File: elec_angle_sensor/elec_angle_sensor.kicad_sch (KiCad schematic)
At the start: 19 parts, among them J1 JST SH, J7 JST SH, U1 AS5600L

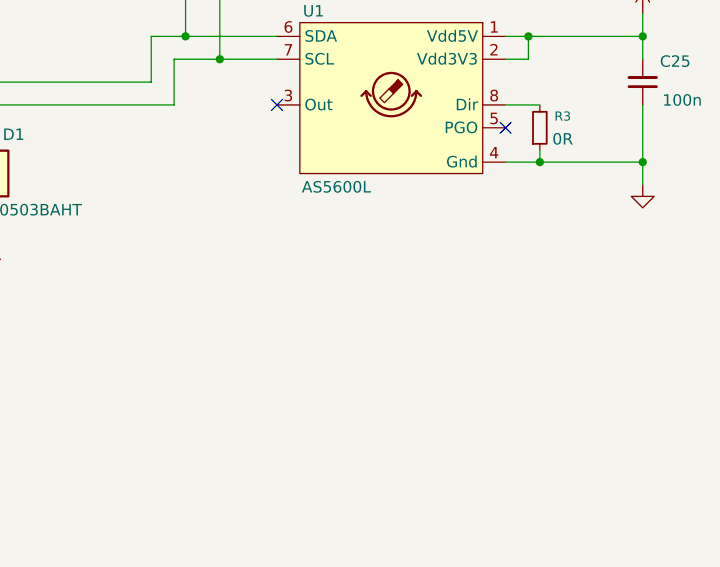
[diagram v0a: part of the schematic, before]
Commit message: [update] Added error to gripette, going to B1
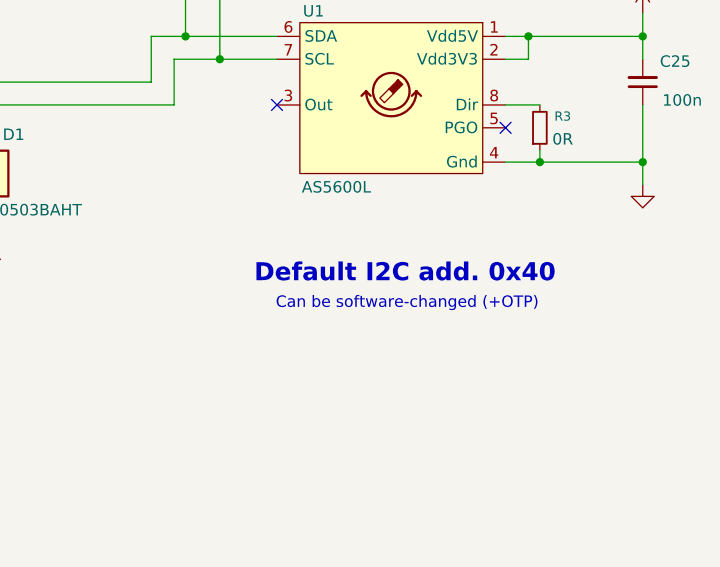
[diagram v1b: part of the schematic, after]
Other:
- note added: "Can be software-changed (+OTP)"
- note added: "Default I2C add. 0x40"
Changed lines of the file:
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@@
+		)
+	)
+	(text "Can be software-changed (+OTP)"
+		(exclude_from_sim no)
+		(at 166.878 131.318 0)
+		(effects
+			(font
+				(size 1.27 1.27)
+			)
 		)
 	)
@@
 		)
 	)
+	(text "Default I2C add. 0x40"
+		(exclude_from_sim no)
+		(at 166.624 128.016 0)
+		(effects
+			(font
+				(size 2 2)
+				(thickness 0.4)
+				(bold yes)
+			)
+		)
+	)
